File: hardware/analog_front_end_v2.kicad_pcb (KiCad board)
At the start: 4 copper layers, 145 x 44 mm, 101 parts, among them J1 Conn_Coaxial, J3 Conn_01x01_Socket, J4 Conn_01x01_Socket, U1 ADL5531, U10 MAX6002, U11 LP2985-5.0, U12 MAX2606, U13 PAT1220-C-0DB, U14 LP2985-5.0, U15 BFP540ESD, U16 BFP540ESD, U17 LP2985-3.3, U18 PAT1220-C-0DB, U19 PAT1220-C-0DB, U2 ADL5531, U20 PAT1220-C-0DB, U21 PAT1220-C-0DB, U3 ADL5531, U4 ADL5531, U5 LP2985-1.8, U6 MCP33131, U7 PAT1220-C-0DB, U8 ADL5531, U9 PMOD 2x6

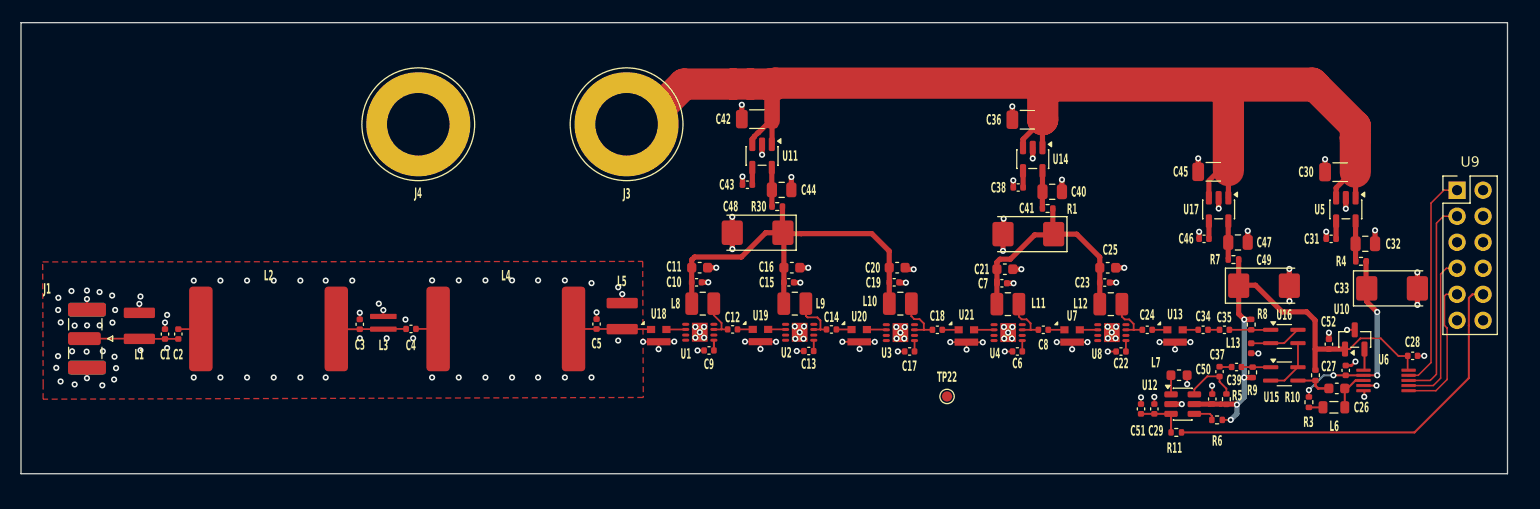
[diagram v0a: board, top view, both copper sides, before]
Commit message: Update prj/sch/pcb files sent off for manufacturing
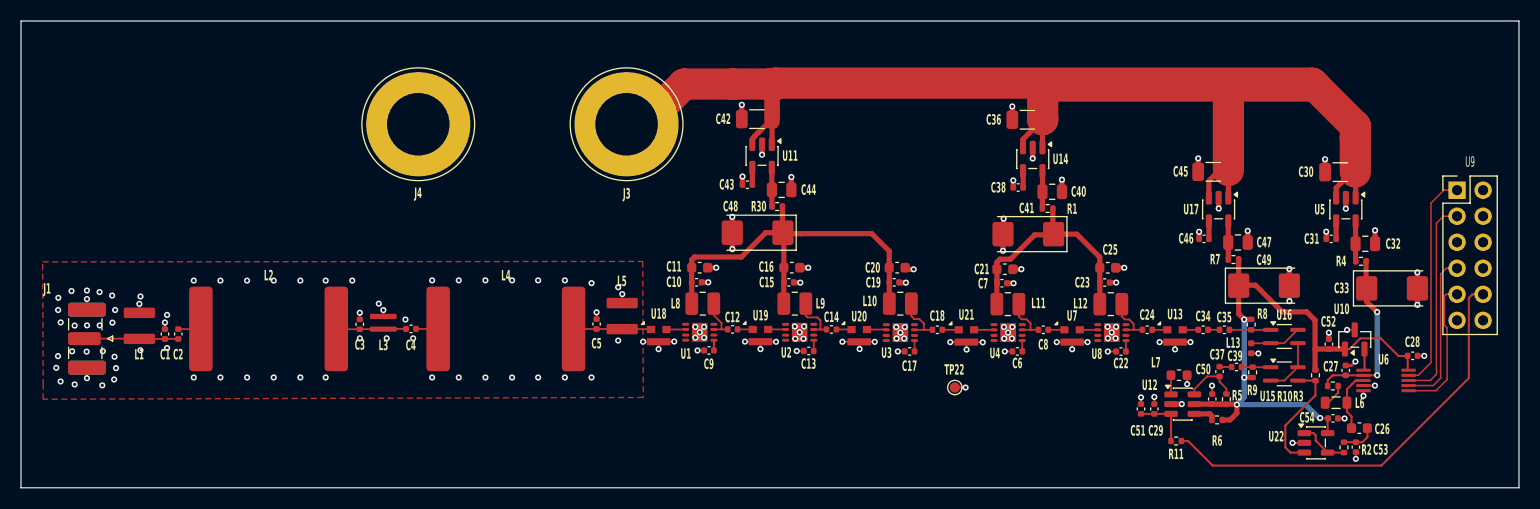
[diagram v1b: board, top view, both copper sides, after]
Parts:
- added C53: 10n_25V, Capacitor_SMD:C_0402_1005Metric, F.Cu at (142.3, 52.0)
- added C54: 100n_25V, Capacitor_SMD:C_0402_1005Metric, F.Cu at (140.0, 49.2)
- added R2: 100, Resistor_SMD:R_0402_1005Metric, F.Cu at (141.1, 52.0)
- added U22: MCP6286, Package_TO_SOT_SMD:SOT-23-5, F.Cu at (138.4, 51.6)
- U9: value PMOD 2x6 -> PMOD 2x6 2.54mm pitch
- moved C26 4.45 mm to (142.6, 50.1), turned to 180 degrees
- moved R3 2.82 mm to (140.0, 46.0), turned to 0 degrees
- moved TP22 1.16 mm to (103.1, 46.2)
- moved R11 0.84 mm to (124.7, 51.4)
- moved L6 0.50 mm to (140.3, 47.7)
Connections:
- C26 pad 1: Net-(U15-C) -> Net-(C26-Pad1)
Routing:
- net 3V3: track 48.4 -> 59.2 mm
- net Net-(U15-C): track 3.63 -> 11.5 mm
- net Net-(U22-Vin-): track 0.00 -> 4.96 mm
- net Net-(C26-Pad1): track 0.00 -> 3.26 mm
- net GND: track 81.1 -> 84.2 mm, vias 163 -> 167
- net PWM_TUNE: track 39.6 -> 41.9 mm
- net 1V8: track 18.8 -> 16.5 mm, vias 4 -> 2
- net Net-(U6-AIN+): track 4.10 -> 5.79 mm
- net Net-(L6-Pad2): track 1.38 -> 2.32 mm
- net Net-(U12-TUNE): track 4.74 -> 5.58 mm
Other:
- board size 145 x 44 mm -> 146.1 x 45.5 mm
- board text added: "Decisions: Dimensions: 146mm x 45.5mm Use Coplanar Waveguide for RF filter section for more confined EM fields Use 0.6x0.3 vias Use 7mil trace for CPW section with 4mil gap to coplanar ground (Standard PCB manufacturer limit) assuming 1ounce copper, 0.1mm high prepreg, 4.6 dielectric constant Use 1mm via distance (2xgap) Use 2mm between vias horizontally Use 7mil for microstrip for around 50ohm i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"
- board text removed: "Decisions: Dimensions: 145mm x 44mm Use Coplanar Waveguide for RF filter section for more confined EM fields Use 0.6x0.3 vias Use 7mil trace for CPW section with 4mil gap to coplanar ground (Standard PCB manufacturer limit) assuming 1ounce copper, 0.1mm high prepreg, 4.6 dielectric constant Use 1mm via distance (2xgap) Use 2mm between vias horizontally Use 7mil for microstrip for around 50ohm imp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"
